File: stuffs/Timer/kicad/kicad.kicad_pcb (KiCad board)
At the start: 2 copper layers, 13 parts, among them CON1 AVR-ISP-6, IC1 ATMEGA328P-P, P1 CONN_01X04, P2 CONN_01X02, SW1 SW_PUSH, SW2 SW_PUSH

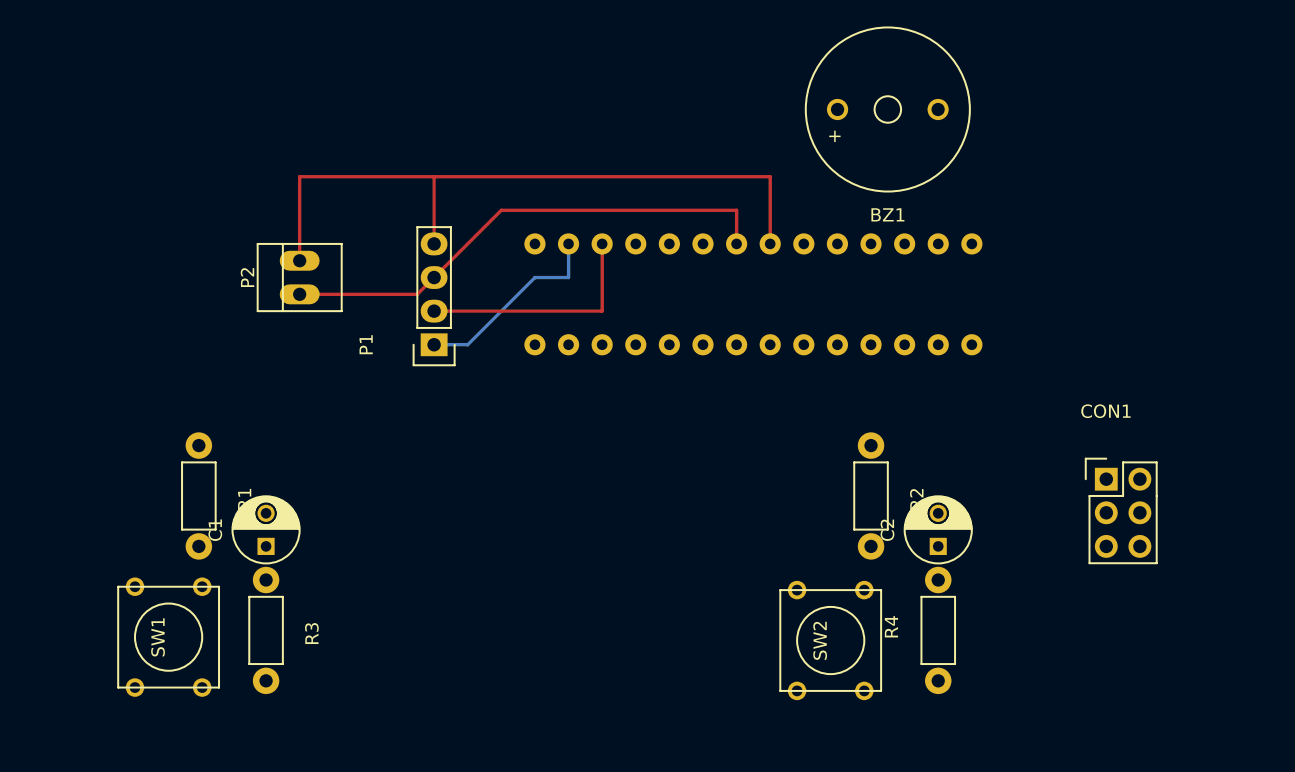
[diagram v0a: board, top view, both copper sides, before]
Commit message: Update kicad design files.
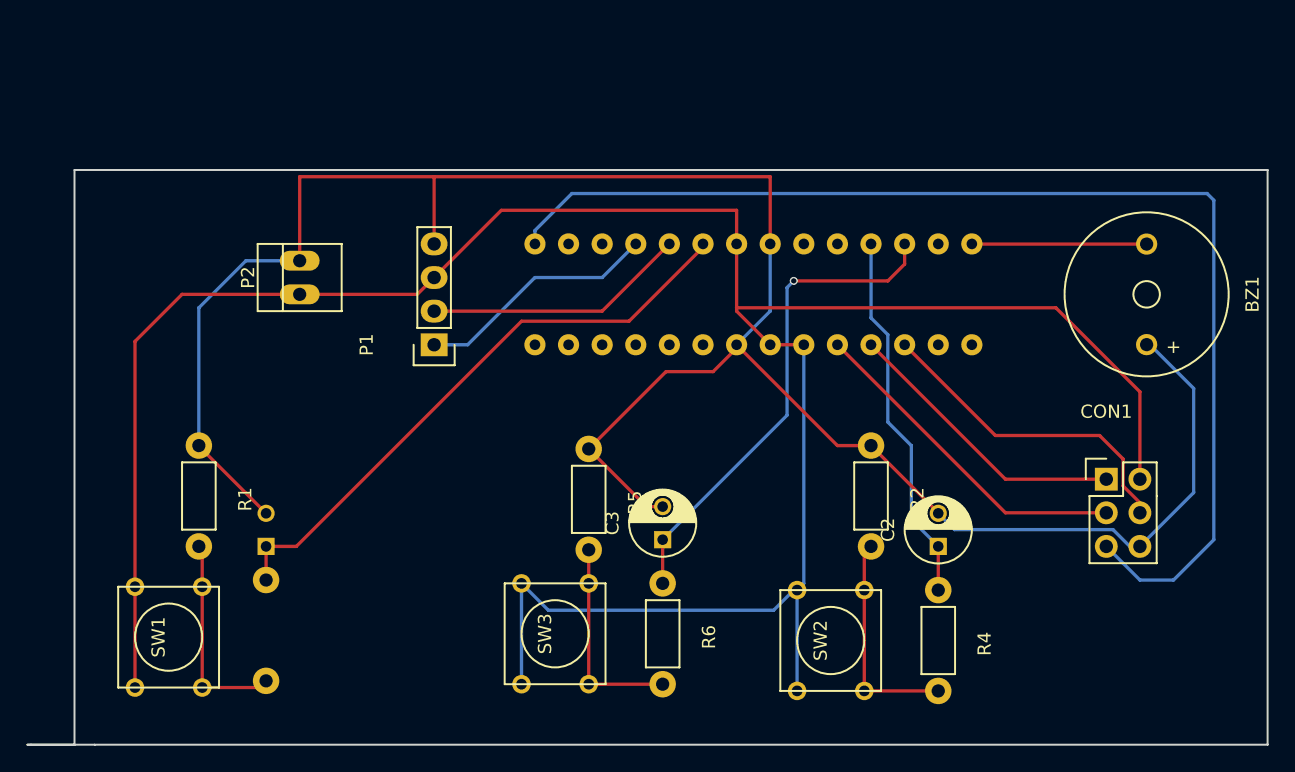
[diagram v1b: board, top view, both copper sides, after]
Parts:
- added C3: 10uF, Capacitors_ThroughHole:C_Radial_D5_L6_P2.5, F.Cu at (121.4, 70.6)
- added R5: 10, Resistors_ThroughHole:Resistor_Horizontal_RM7mm, F.Cu at (115.8, 63.8)
- added R6: 1K, Resistors_ThroughHole:Resistor_Horizontal_RM7mm, F.Cu at (121.4, 73.9)
- added SW3: SW_PUSH, Buttons_Switches_ThroughHole:SW_PUSH_SMALL, F.Cu at (113.3, 77.7)
- C1, R3: moved to B.Cu
- moved BZ1 18.7 mm to (158.0, 48.3), turned to 270 degrees
- moved R4 6.86 mm to (142.2, 74.4), turned to 270 degrees
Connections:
- IC1 pad 11: Net-(IC1-Pad11) -> INCREASE
- IC1 pad 12: Net-(IC1-Pad12) -> DECREASE
- IC1 pad 2: DISPLAY_CLK -> Net-(IC1-Pad2)
- IC1 pad 3: DISPLAY_IO -> Net-(IC1-Pad3)
- IC1 pad 4: PLAY -> DISPLAY_CLK
- IC1 pad 5: Net-(IC1-Pad5) -> DISPLAY_IO
- IC1 pad 6: Net-(IC1-Pad6) -> PLAY
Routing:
- net VCC: track 38.2 -> 185.5 mm
- net GND: track 52.1 -> 164.8 mm
- net Net-(CON1-Pad5): track 0.00 -> 89.8 mm
- net PLAY: track 0.00 -> 45.2 mm
- net DECREASE: track 0.00 -> 37.4 mm, vias 0 -> 1
- net INCREASE: track 0.00 -> 28.3 mm
- net Net-(CON1-Pad3): track 0.00 -> 25.6 mm
- net Net-(CON1-Pad4): track 0.00 -> 25.2 mm
- net Net-(CON1-Pad1): track 0.00 -> 22.0 mm
- net Net-(R2-Pad2): track 0.00 -> 16.7 mm
- net Net-(R1-Pad2): track 0.00 -> 15.8 mm
- net Net-(R5-Pad2): track 0.00 -> 15.7 mm
- net Net-(BZ1-Pad1): track 0.00 -> 13.2 mm
- net DISPLAY_CLK: track 14.8 -> 18.4 mm
- net DISPLAY_IO: track 17.8 -> 19.9 mm
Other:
- board outline added: 93.7 x 43.4 mm
